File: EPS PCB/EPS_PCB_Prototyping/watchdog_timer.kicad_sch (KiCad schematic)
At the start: 5 parts, among them U4 TPS3431SDRBR

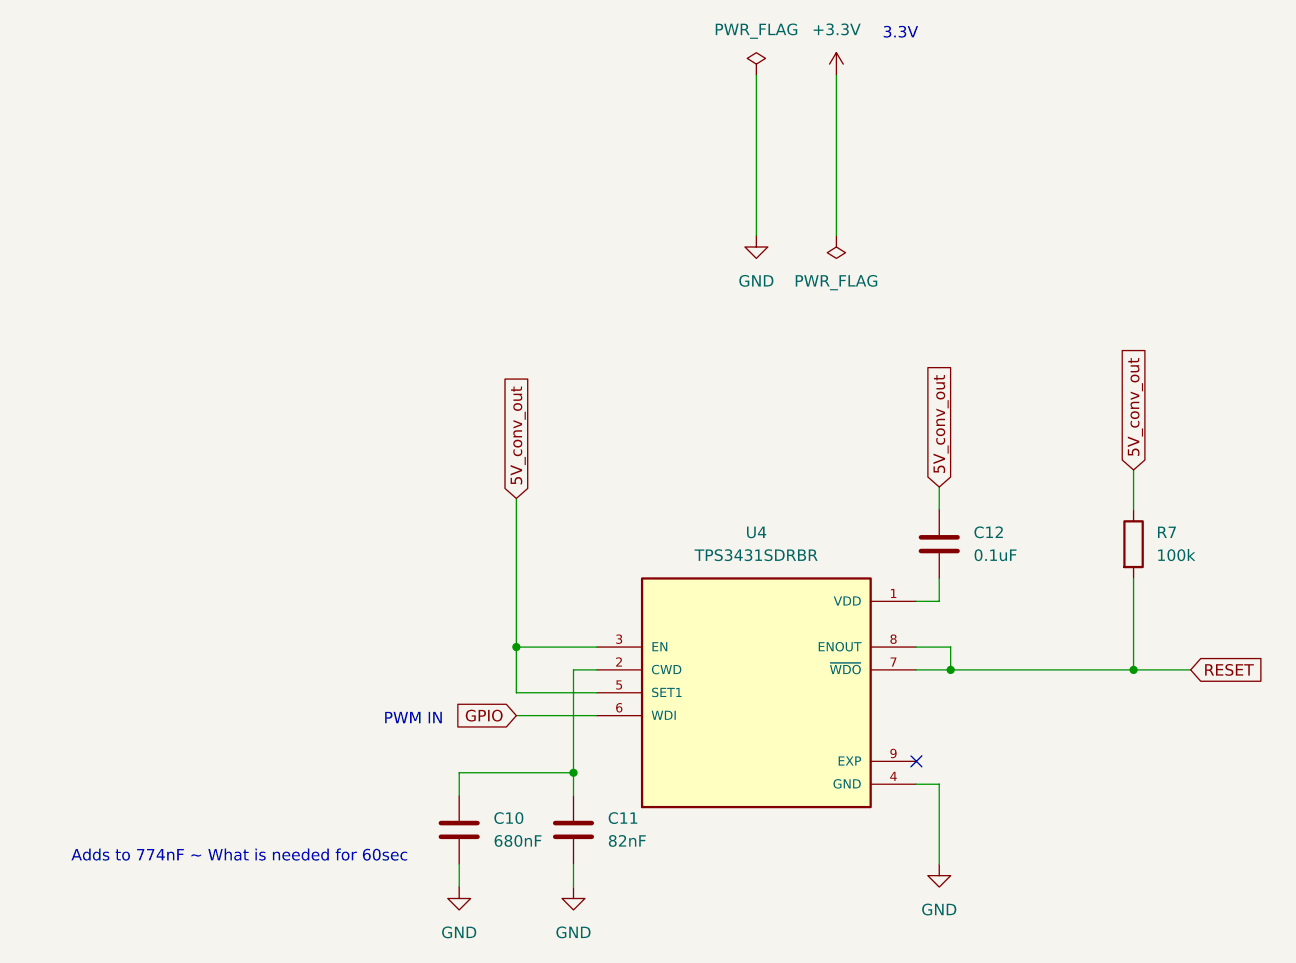
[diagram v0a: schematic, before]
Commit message: EPS PCB Prototype For order
yea
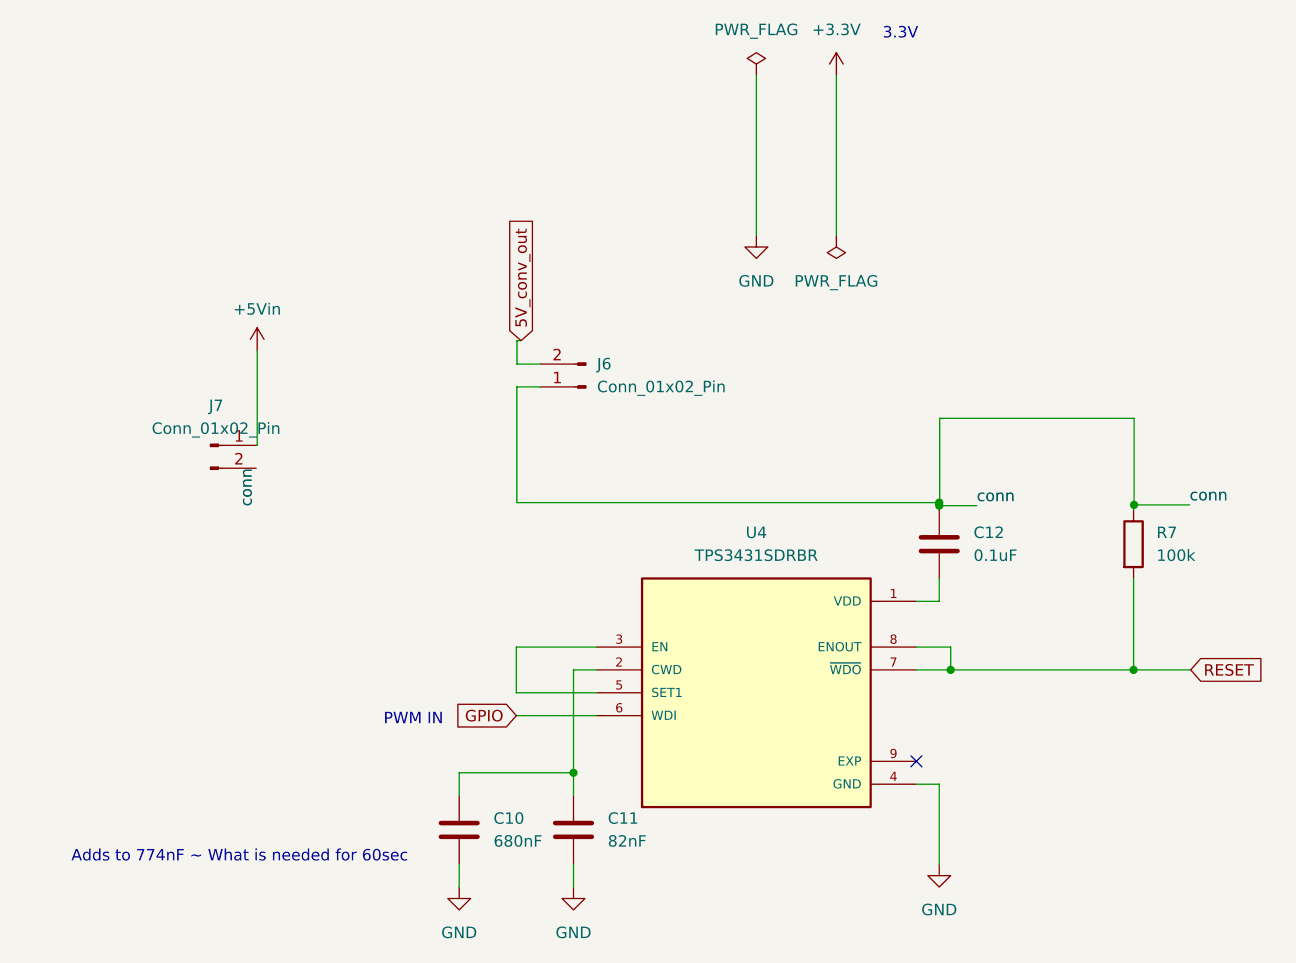
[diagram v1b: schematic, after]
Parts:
- added J6, J7: Conn_01x02_Pin, Connector_PinSocket_2.54mm:PinSocket_1x02_P2.54mm_Vertical, symbol Connector:Conn_01x02_Pin
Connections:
- net 5V_conv_out: now also J6.2 (Pin_2); no longer C12.1, R7.1, U4.3 (EN), U4.5 (SET1)
- new net: U4.3 (EN), U4.5 (SET1)
- new net +5Vin: J7.1 (Pin_1)
- new net conn: C12.1, J6.1 (Pin_1), J7.2 (Pin_2), R7.1
